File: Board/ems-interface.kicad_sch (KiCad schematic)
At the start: 51 parts, among them J8 EMS, Q1 BC858, Q11 BC848, U2 LM393, U3 MP1584

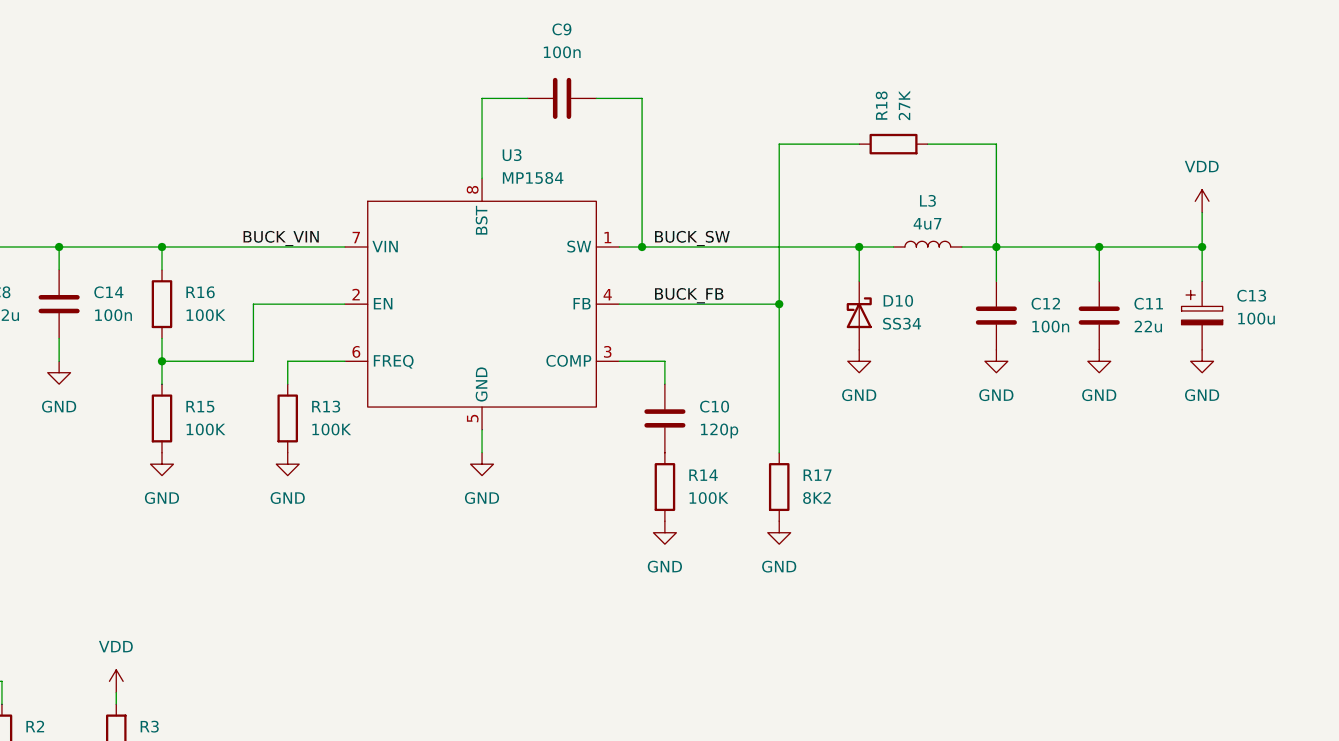
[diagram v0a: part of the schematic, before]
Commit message: Minor fixes
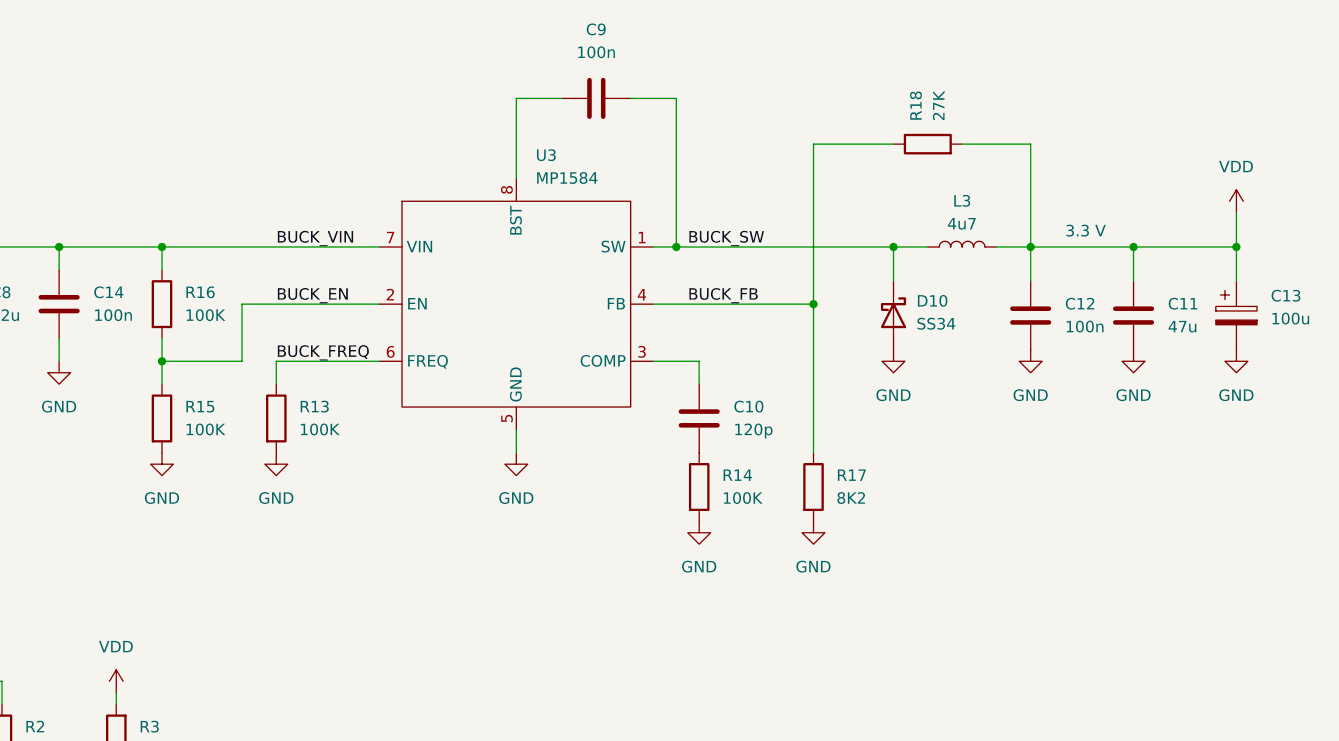
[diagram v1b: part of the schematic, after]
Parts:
- C11: value 22u -> 47u
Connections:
- net BUCK_EN: now reaches R15.1, R16.2, U3.2 (EN)
- net BUCK_FREQ: now reaches R13.1, U3.6 (FREQ)
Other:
- note added: "3.3 V"
- moved on the sheet: C10, C11, C12, C13, C9, D10, L3, R13, R14, R17, R18, U3
